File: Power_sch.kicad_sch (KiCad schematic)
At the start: 36 parts, among them J1 USB4105-GF-A, J2 USB4105-GF-A, U2 TPD2EUSB30ADRTR, U6 ADP150WACBZ-3.3-R7, U7 IR3883MTRPBF

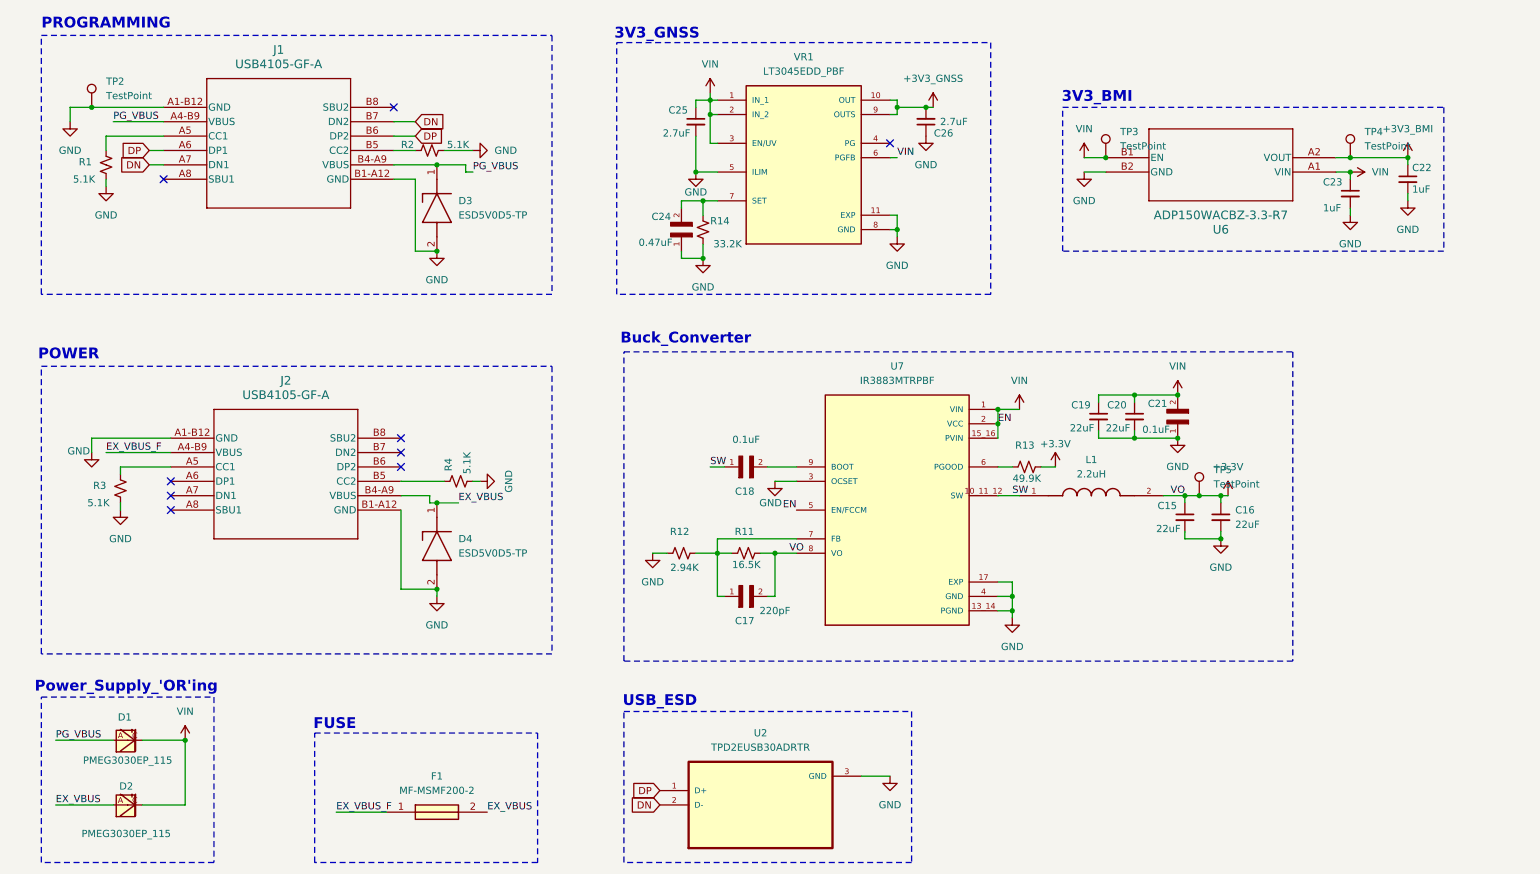
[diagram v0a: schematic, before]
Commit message: new
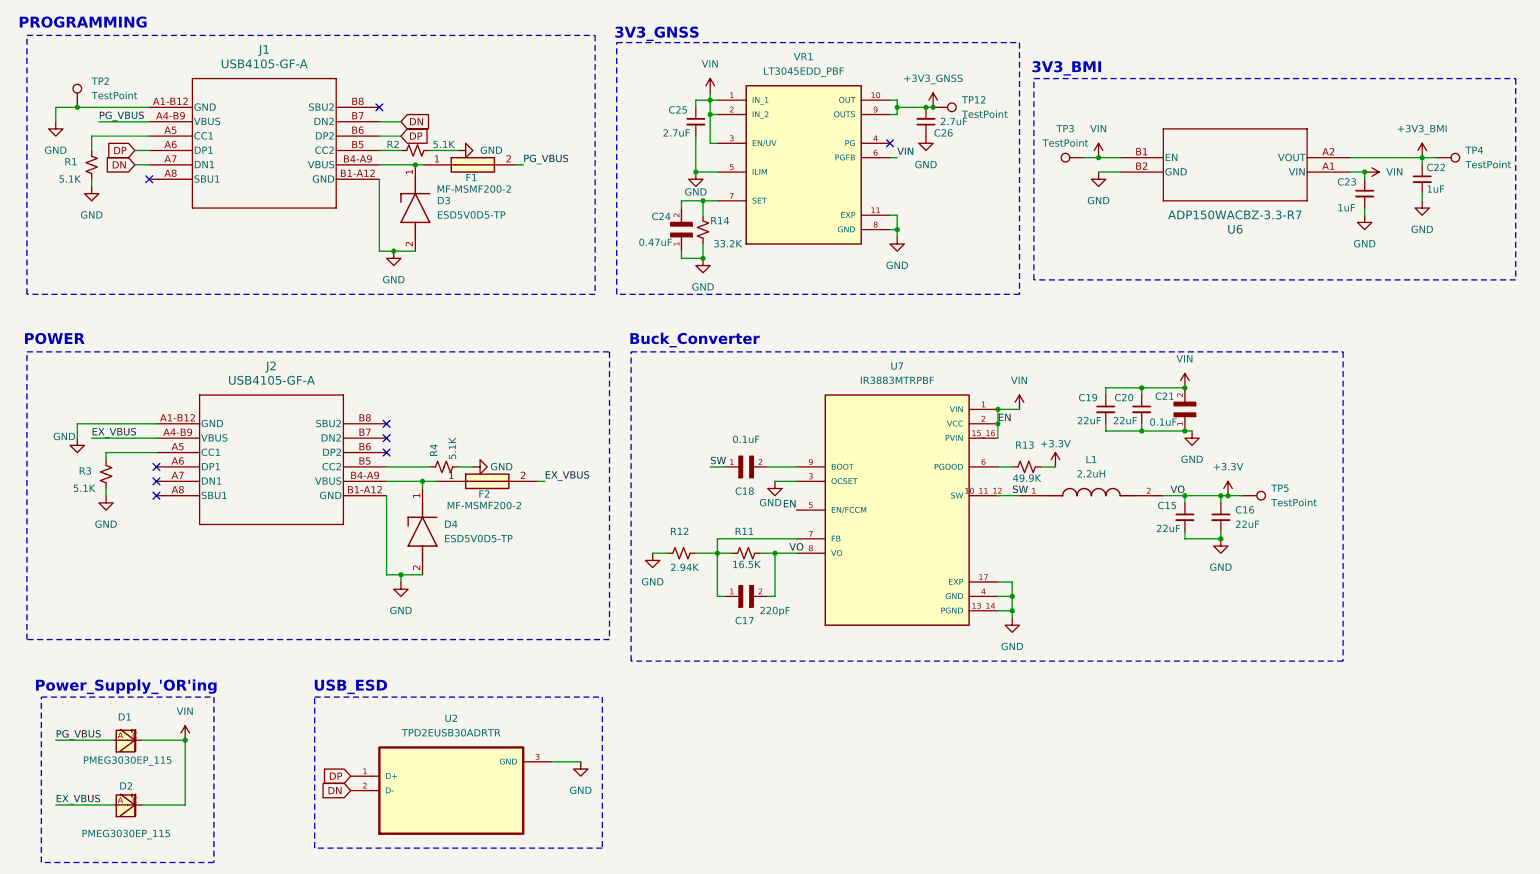
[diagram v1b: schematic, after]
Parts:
- added F2: MF-MSMF200-2, FUSC4632X85N, symbol MF-MSMF200-2:MF-MSMF200-2
- added TP12: TestPoint, TestPoint:TestPoint_Pad_D2.0mm, symbol Connector:TestPoint
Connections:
- net +3V3_GNSS: now also TP12.1
- net EX_VBUS: now also J2.A4-B9 (VBUS), F2.2; no longer D4.1 (K), F1.2, J2.B4-A9 (VBUS)
- net PG_VBUS: now also F1.2; no longer D3.1 (K), J1.B4-A9 (VBUS)
- net EX_VBUS_F: no longer names the net of F1.1
- net EX_VBUS_F: now also D3.1 (K), J1.B4-A9 (VBUS); no longer J2.A4-B9 (VBUS)
- new net: D4.1 (K), F2.1, J2.B4-A9 (VBUS)
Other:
- note removed: "FUSE"
- moved on the sheet: C19, C20, C21, C22, C23, D3, D4, F1, J1, J2, R1, R2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
